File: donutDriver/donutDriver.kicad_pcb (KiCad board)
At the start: 2 copper layers, 13 x 19 mm, 42 parts, among them J1 Keystone 7767, J2 Keystone 7767, J3 Keystone 7767, J4 Keystone 7767, J5 Keystone 7767, J6 Conn_Coaxial_Small, J7 Conn_Coaxial_Small, Q1 IPP320N20N3, Q2 BSS138

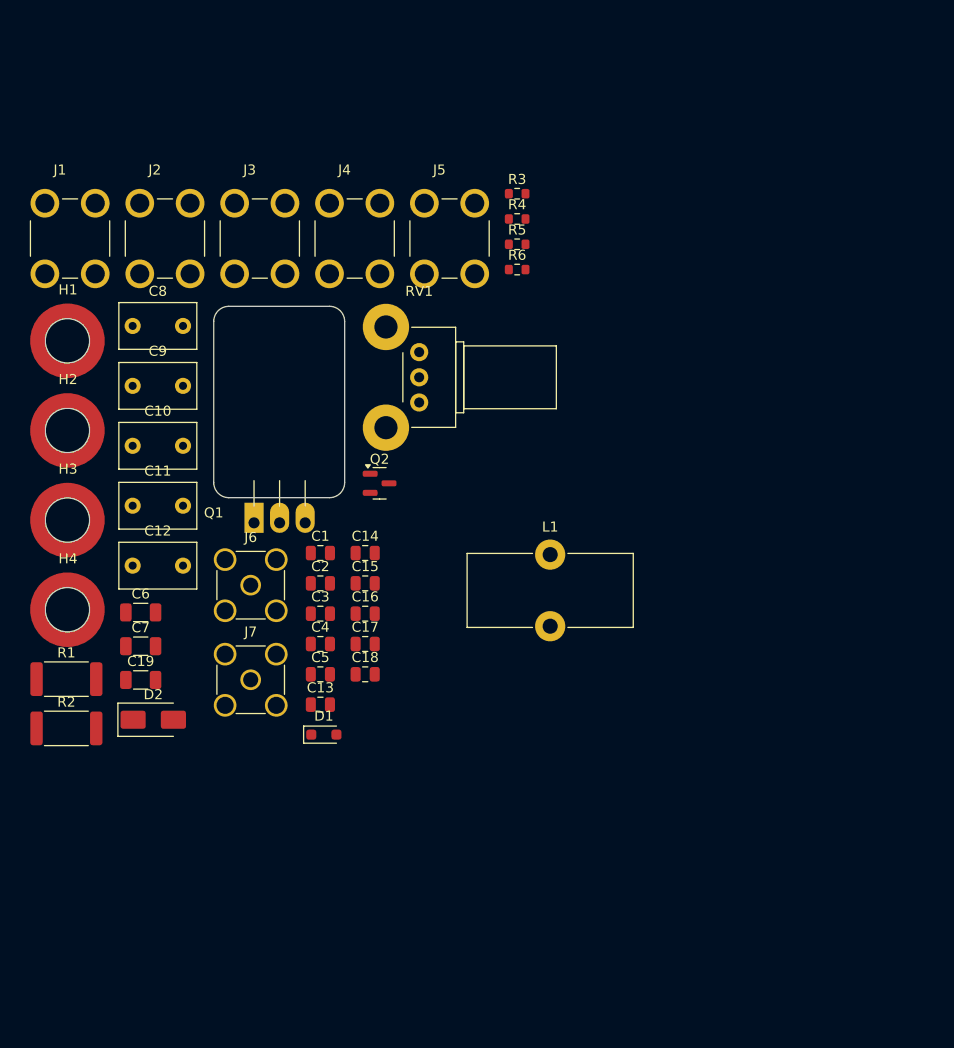
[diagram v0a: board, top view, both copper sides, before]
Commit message: begin pcb
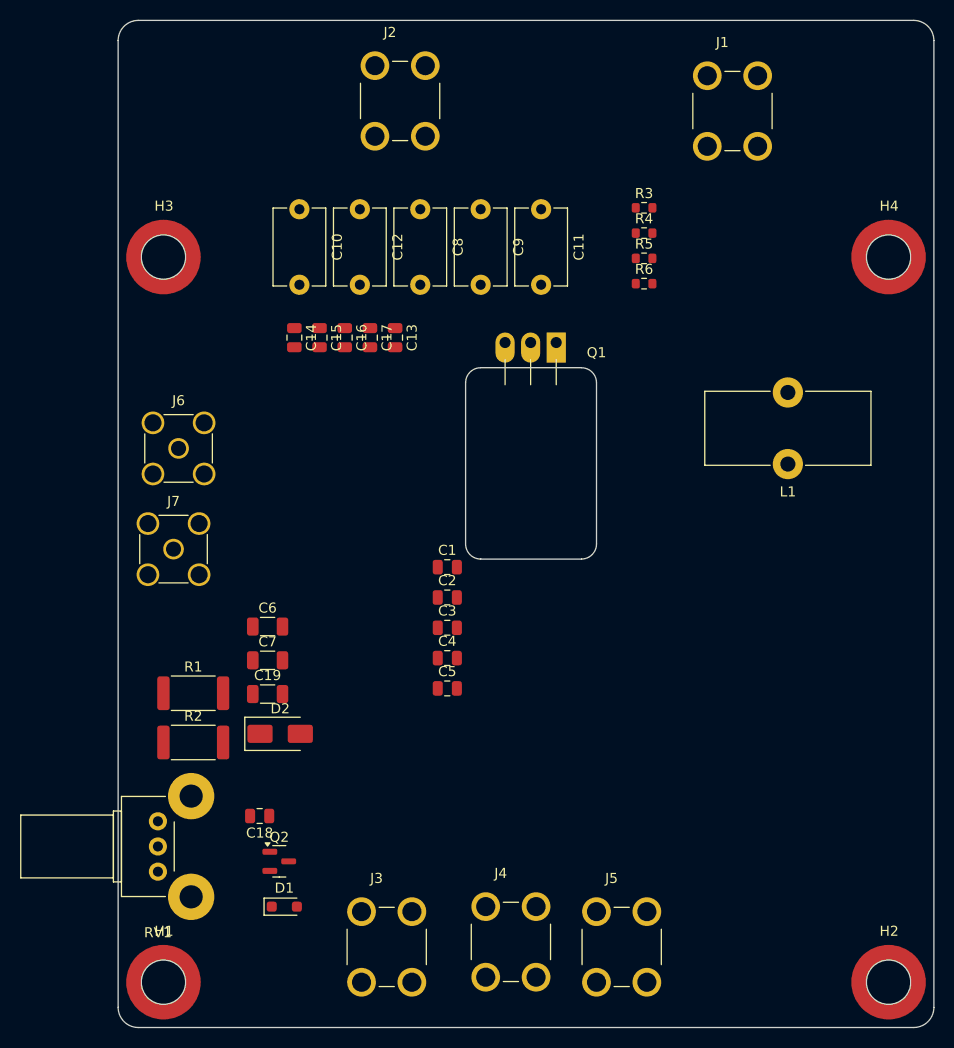
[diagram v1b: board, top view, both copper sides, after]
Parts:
- C10, C11, C12, C8, C9: footprint Capacitor_THT:C_Disc_D7.5mm_W4.4mm_P5.00mm -> donutlib:TDK_Disc_D7.5mm_W5.0mm_P7.50mm
- moved H2 98.2 mm to (176.5, 145.5)
- moved H4 88.7 mm to (176.5, 73.5)
- moved J5 72.4 mm to (150.0, 142.0)
- moved J4 71.5 mm to (139.0, 141.5)
- moved J3 71.5 mm to (126.7, 142.0)
- moved J1 67.0 mm to (161.0, 59.0)
- moved H1 64.4 mm to (104.5, 145.5)
- moved C11 50.1 mm to (142.0, 68.8), turned to -90 degrees
- moved RV1 49.0 mm to (104.0, 129.5), turned to 180 degrees
- moved C12 42.0 mm to (124.0, 68.8), turned to -90 degrees
- moved Q2 38.8 mm to (116.0, 133.5)
- moved C9 38.8 mm to (136.0, 68.8), turned to -90 degrees
- moved C13 37.2 mm to (127.5, 81.5), turned to -90 degrees
- moved Q1 34.4 mm to (143.5, 82.5), turned to 180 degrees
- moved C8 30.8 mm to (130.0, 68.8), turned to -90 degrees
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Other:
- board size 13 x 19 mm -> 81 x 100 mm
